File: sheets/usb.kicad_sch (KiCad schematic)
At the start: 9 parts, among them U2 USBLC6-2SC6, U4 AP7384-33SA

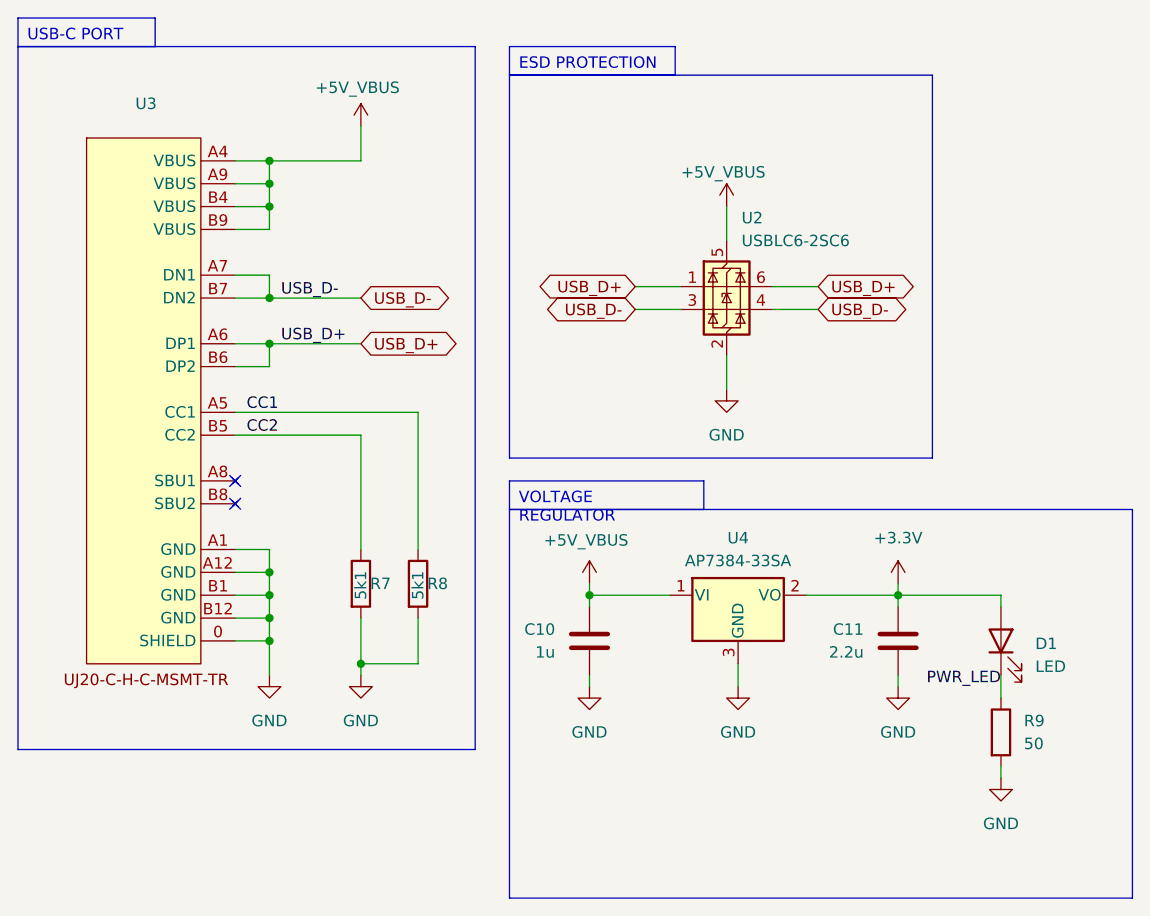
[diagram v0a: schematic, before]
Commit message: dasdsad
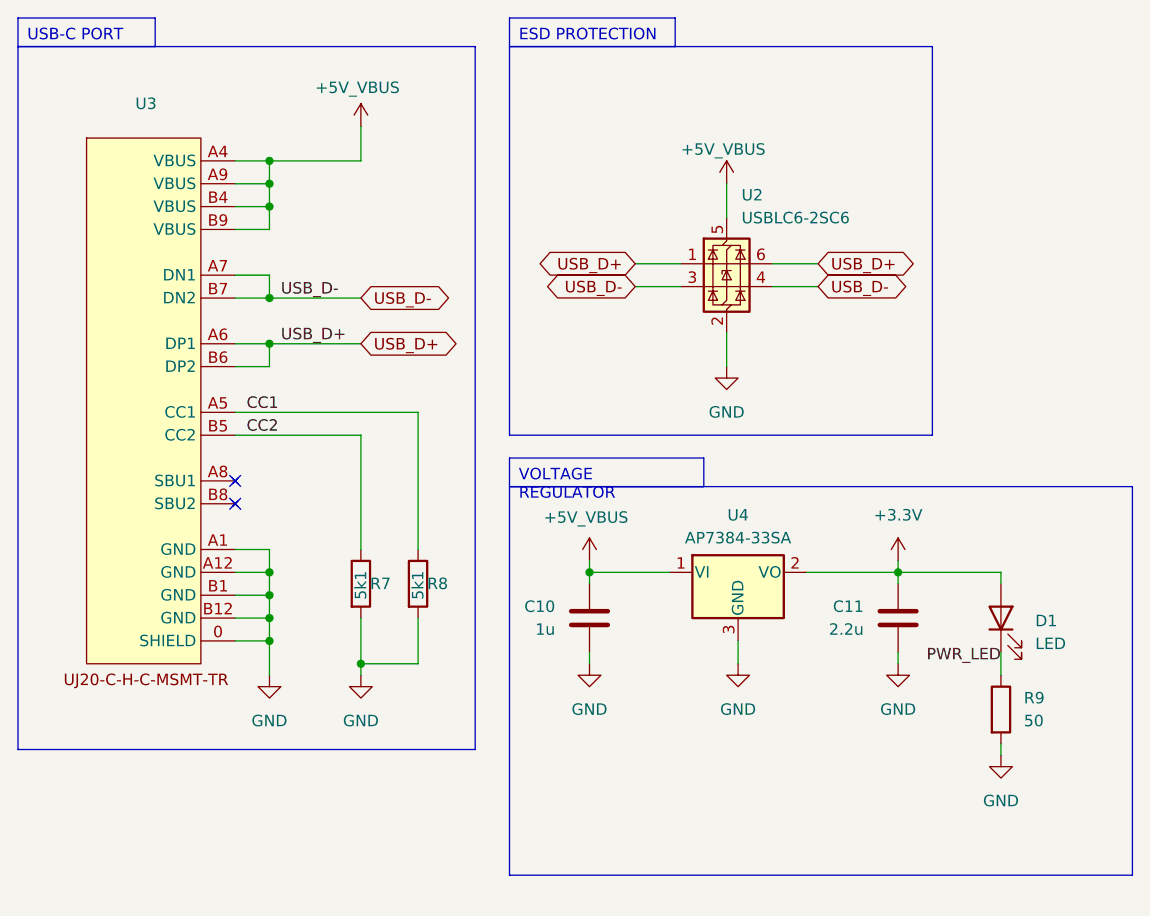
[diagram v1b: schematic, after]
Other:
- moved on the sheet: C10, C11, D1, R9, U2, U4
